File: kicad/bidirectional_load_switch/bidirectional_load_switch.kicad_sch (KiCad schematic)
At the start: 28 parts, among them J101 1017503, J102 Conn_01x09_Socket, J103 Conn_01x02_Socket, J104 Conn_01x02_Socket, J105 Conn_01x02_Socket, J106 Conn_01x02_Socket, J107 AVR-ISP-6, SW101 PTS526 SK15 SMTR2 LFS, U101 TMCS1101A3BQDR, U102 TLV75733PDBVR, U104 ATTINY85-20SU

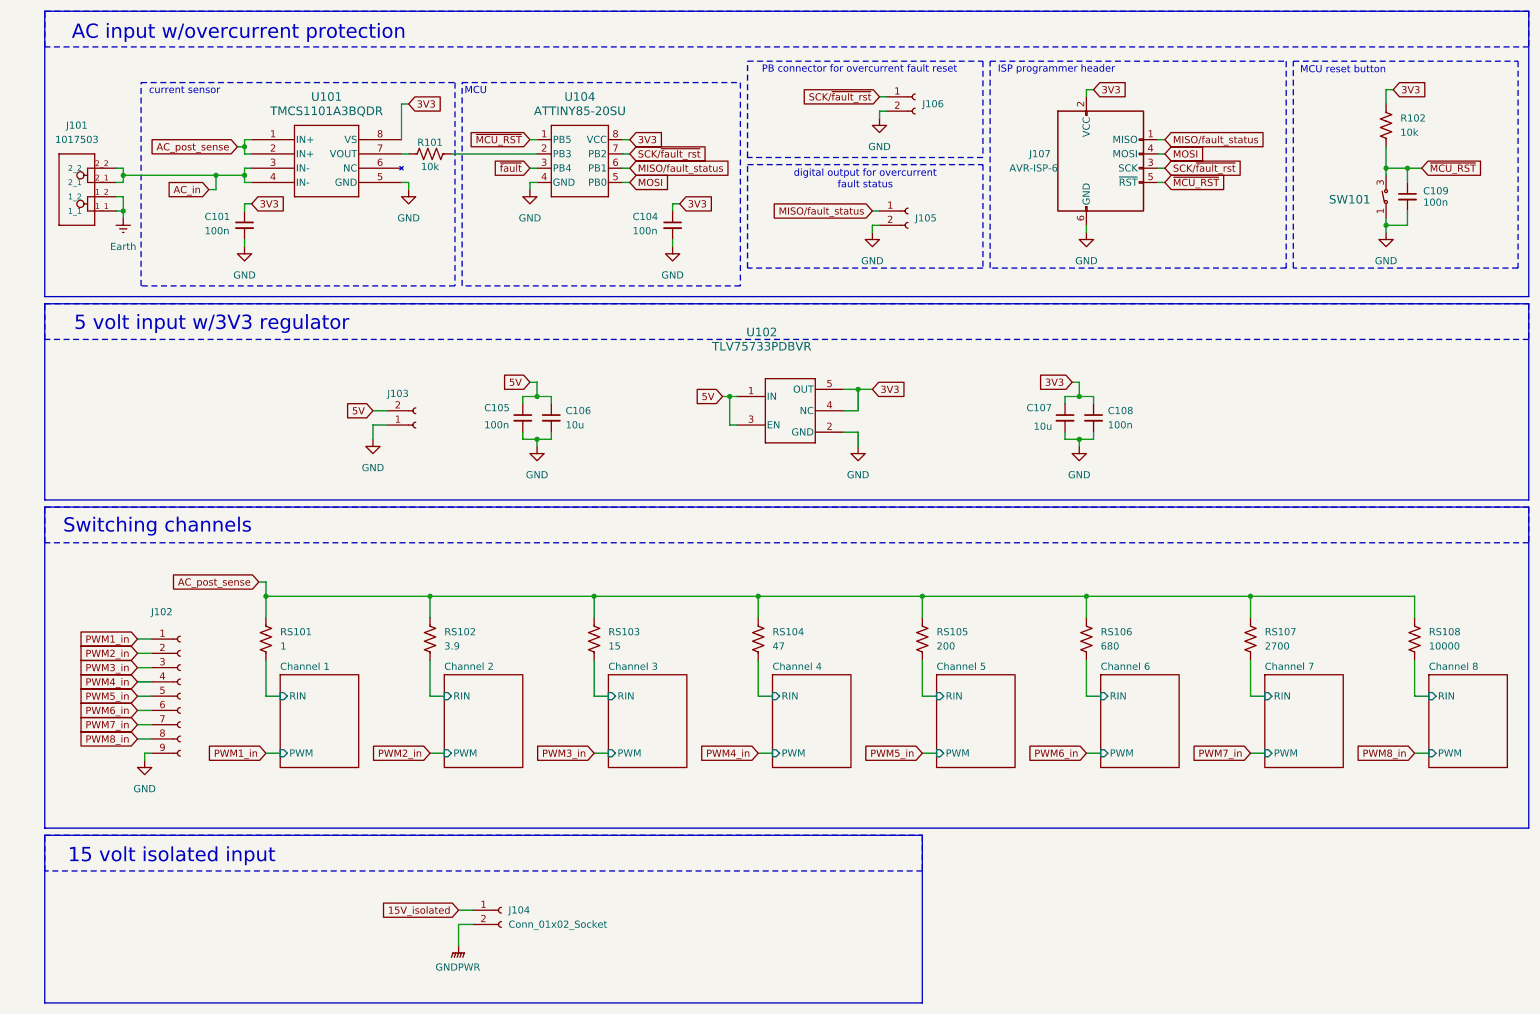
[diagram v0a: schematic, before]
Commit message: almost
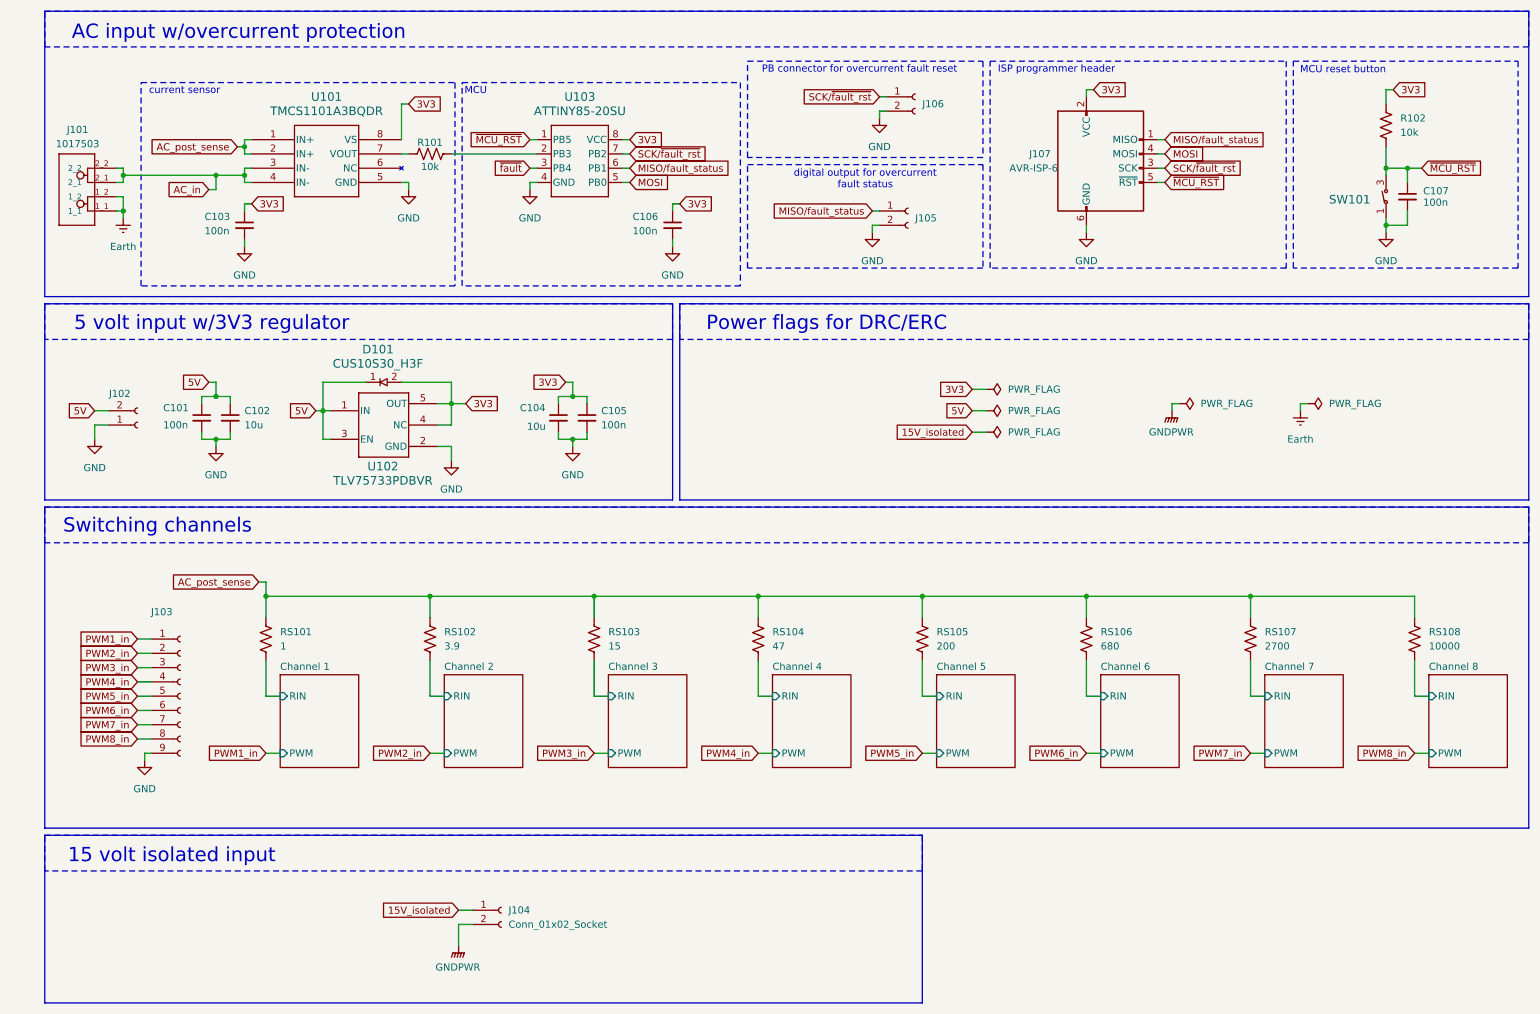
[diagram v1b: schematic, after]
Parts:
- added D101: CUS10S30_H3F, diode_CUS10S30_H3F:USC_TOS, symbol diode_CUS10S30_H3F:CUS10S30_H3F
- U102: footprint DBV0005A_N -> ldo_TLV75733PDBVR:DBV0005A_L
- renumbered C105 to C101, C106 to C102, C101 to C103, C107 to C104, C108 to C105, C104 to C106, C109 to C107, J103 to J102, J102 to J103, U104 to U103
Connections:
- net 3V3: now also D101.2
- net 5V: now also D101.1
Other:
- note added: "Power flags for DRC/ERC"
- moved on the sheet: C101, C102, C104, C105, J102, U102

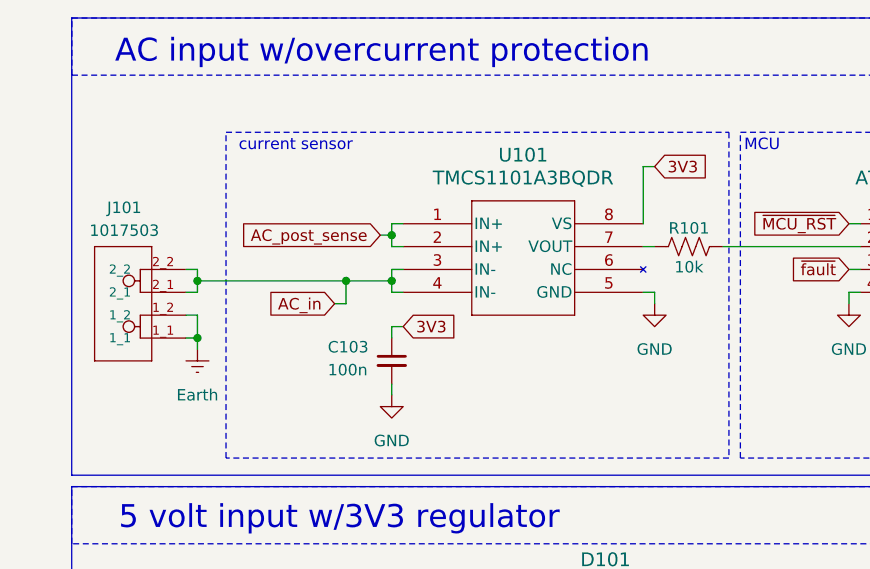
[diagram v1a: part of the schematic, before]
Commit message: needs review
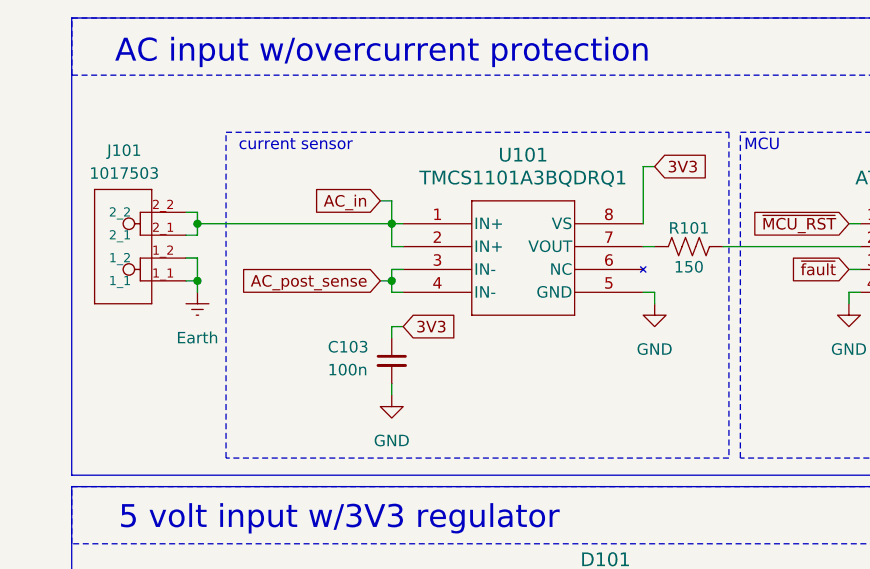
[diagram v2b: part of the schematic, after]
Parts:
- R101: value 10k -> 150
- SW101: footprint switch_switch_PTS526_SK15_SMTR2_LFS:SMT_FS -> switch_PTS526_SK15_SMTR2_LFS:SMT_FS
- U101: value TMCS1101A3BQDR -> TMCS1101A3BQDRQ1
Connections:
- net AC_in: now also U101.1 (IN+), U101.2 (IN+); no longer U101.3 (IN-), U101.4 (IN-)
- net AC_post_sense: now also U101.3 (IN-), U101.4 (IN-); no longer U101.1 (IN+), U101.2 (IN+)
